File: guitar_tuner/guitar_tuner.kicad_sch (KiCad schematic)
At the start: 0 parts

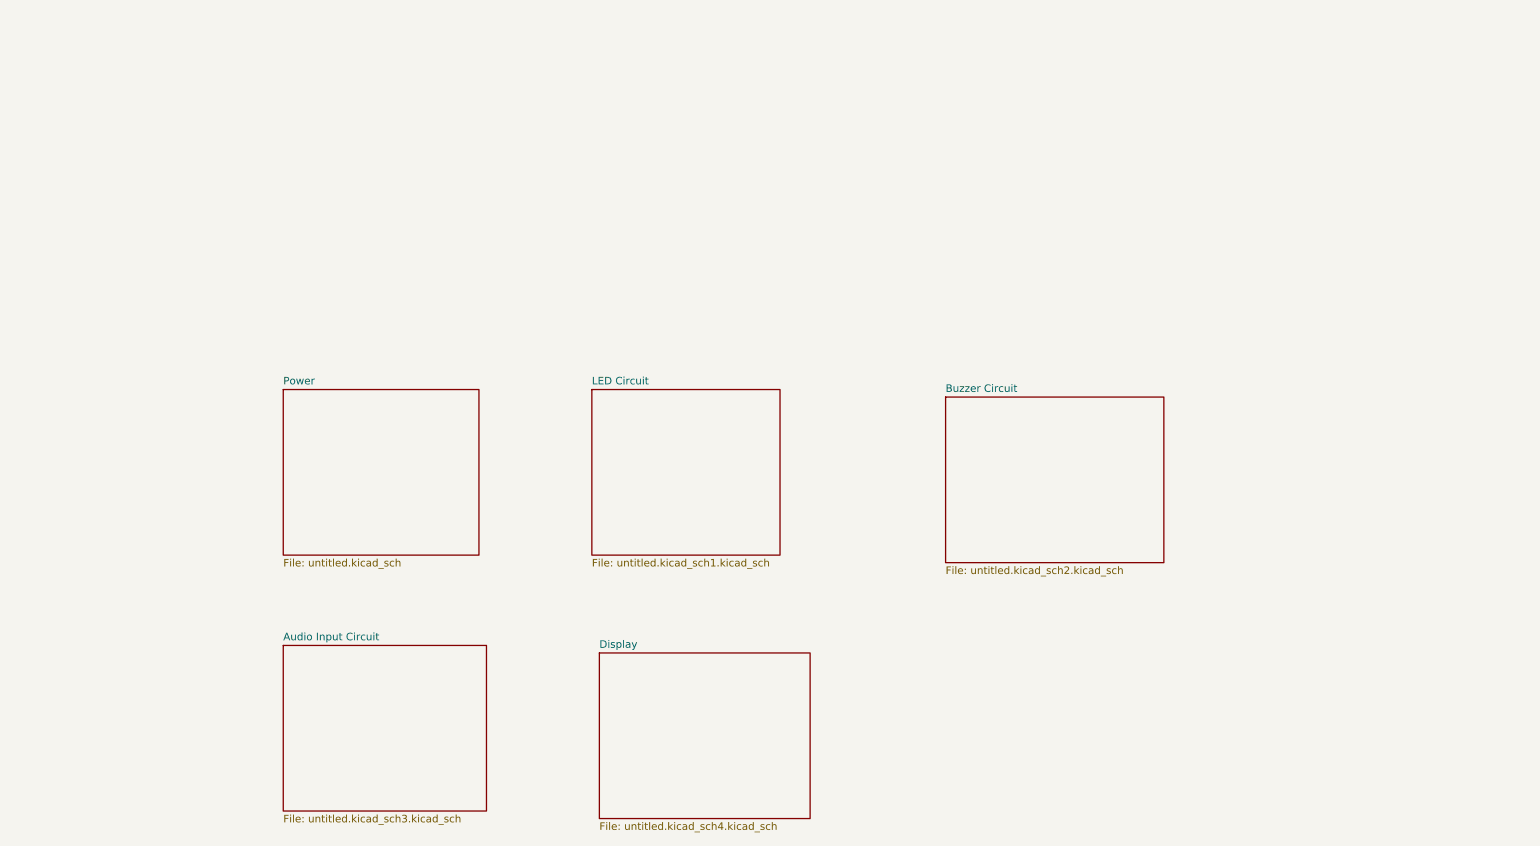
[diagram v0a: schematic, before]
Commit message: ESP32
ESP32 Addition
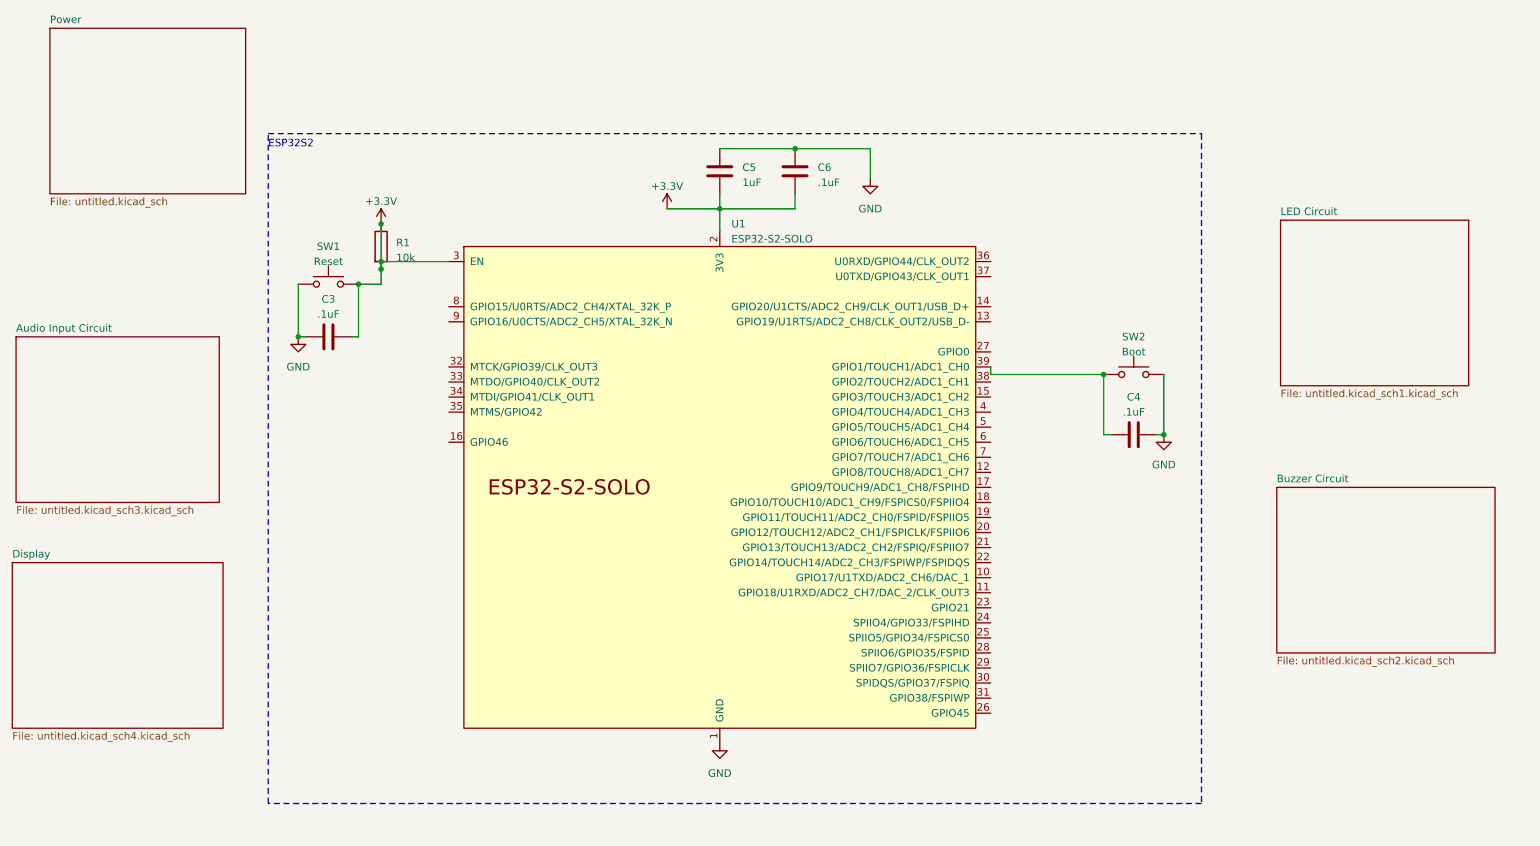
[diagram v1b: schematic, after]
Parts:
- added C3, C4, C6: .1uF, symbol Device:C
- added C5: 1uF, symbol Device:C
- added R1: 10k, symbol Device:R
- added SW1: Reset, symbol Switch:SW_Omron_B3FS
- added SW2: Boot, symbol Switch:SW_Omron_B3FS
- added U1: ESP32-S2-SOLO, PCM_Espressif:ESP32-S2-SOLO, symbol esp32:ESP32-S2-SOLO
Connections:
- new net: C4.1, SW2.1, U1.39 (GPIO1/TOUCH1/ADC1_CH0)
- new net +3.3V: C3.2, C5.2, C6.2, R1.1, R1.2, SW1.2, U1.2 (3V3), U1.3 (EN)
- new net GND: C3.1, C4.2, C5.1, C6.1, SW1.1, SW2.2, U1.1 (GND), U1.40 (GND), U1.41 (GND)
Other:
- note added: "ESP32S2"
